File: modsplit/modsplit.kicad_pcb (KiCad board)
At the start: 2 copper layers, 19 x 19 mm, 8 parts, among them J1 Conn_01x04, J2 Conn_01x04, J3 Conn_01x04, J4 Conn_01x04, U1 TRRS, U2 TRRS, U3 TRRS, U4 TRRS

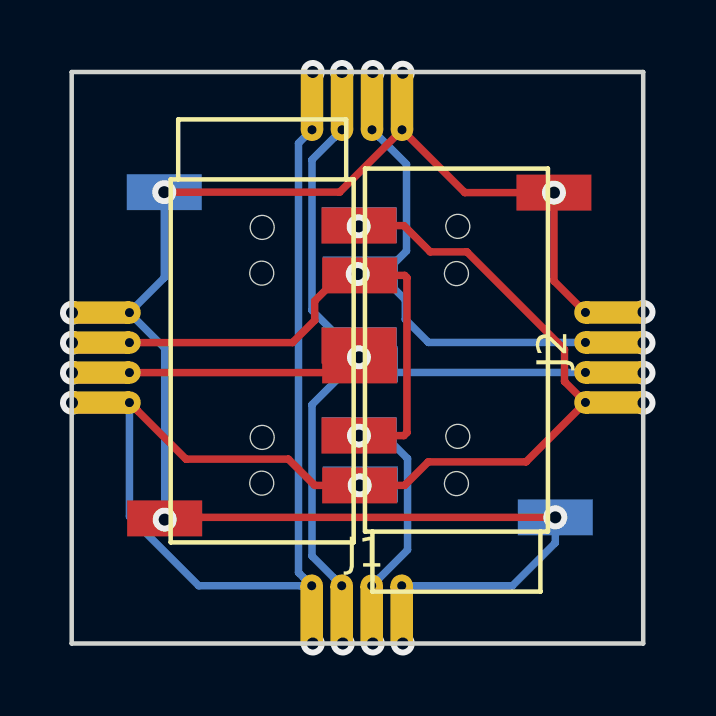
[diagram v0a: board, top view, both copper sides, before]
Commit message: pull up with less than the force of a thousand suns
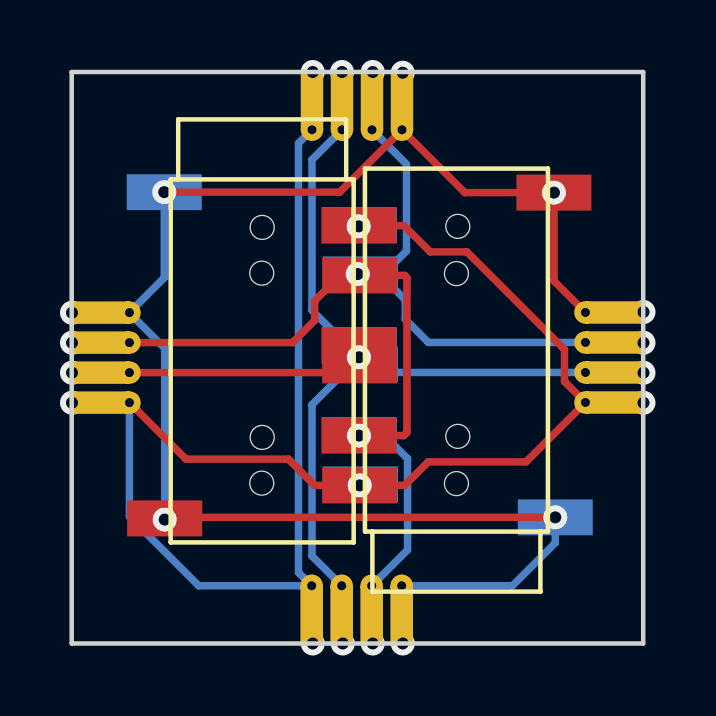
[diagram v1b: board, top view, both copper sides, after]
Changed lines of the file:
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@@
   (module Keebio-Parts:TRRS-PJ-320D (layer B.Cu)
     (at 133.585 89.765 180)
-    (fp_text reference U4 (at 0 -14.2) (layer Dwgs.User)
+    (fp_text reference U4 (at 0 -14.2) (layer Dwgs.User) hide
       (effects (font (size 1 1) (thickness 0.15)))
     )
@@
   (module Keebio-Parts:TRRS-PJ-320D (layer F.Cu)
     (at 133.54 101.54 180)
-    (fp_text reference U3 (at 0 14.2) (layer Dwgs.User)
+    (fp_text reference U3 (at 0 14.2) (layer Dwgs.User) hide
       (effects (font (size 1 1) (thickness 0.15)))
     )
@@
   (module Keebio-Parts:TRRS-PJ-320D (layer F.Cu)
     (at 127.065 89.8)
-    (fp_text reference U2 (at 0 14.2) (layer Dwgs.User)
+    (fp_text reference U2 (at 0 14.2) (layer Dwgs.User) hide
       (effects (font (size 1 1) (thickness 0.15)))
     )
@@
   (module Keebio-Parts:TRRS-PJ-320D (layer B.Cu)
     (at 127.05 101.525)
-    (fp_text reference U1 (at 0 -14.2) (layer Dwgs.User)
+    (fp_text reference U1 (at 0 -14.2) (layer Dwgs.User) hide
       (effects (font (size 1 1) (thickness 0.15)))
     )
@@
   (module modkeeb:edgeconnector (layer B.Cu)
     (at 130.225 86.145)
-    (fp_text reference J4 (at 0.275 3.1 180) (layer B.SilkS)
+    (fp_text reference J4 (at 0.275 3.1 180) (layer B.SilkS) hide
       (effects (font (size 1 1) (thickness 0.15)) (justify mirror))
     )
@@
   (module modkeeb:edgeconnector (layer B.Cu)
     (at 120.64 95.74 90)
-    (fp_text reference J3 (at 0.275 3.1 90) (layer B.SilkS)
+    (fp_text reference J3 (at 0.275 3.1 90) (layer B.SilkS) hide
       (effects (font (size 1 1) (thickness 0.15)) (justify mirror))
     )
@@
   (module modkeeb:edgeconnector (layer F.Cu)
     (at 139.84 95.735 90)
-    (fp_text reference J2 (at 0.275 -3.1 270) (layer F.SilkS)
+    (fp_text reference J2 (at 0.275 -3.1 270) (layer F.SilkS) hide
       (effects (font (size 1 1) (thickness 0.15)))
     )
@@
   (module modkeeb:edgeconnector (layer F.Cu)
     (at 130.215 105.345)
-    (fp_text reference J1 (at 0.275 -3.1 180) (layer F.SilkS)
+    (fp_text reference J1 (at 0.275 -3.1 180) (layer F.SilkS) hide
       (effects (font (size 1 1) (thickness 0.15)))
     )
@@
   (gr_line (start 120.715 105.27) (end 120.715 86.22) (layer Edge.Cuts) (width 0.15))
   (gr_line (start 120.715 86.22) (end 139.765 86.22) (layer Edge.Cuts) (width 0.15))
-  (via (at 130.25 92.955) (size 0.8) (drill 0.4) (layers F.Cu B.Cu) (net 2))
-  (via (at 128.75 86.22) (size 0.8) (drill 0.4) (layers F.Cu B.Cu) (net 4))
-  (via (at 120.725 97.245) (size 0.8) (drill 0.4) (layers F.Cu B.Cu) (net 4))
   (via (at 139.775 94.22) (size 0.8) (drill 0.4) (layers F.Cu B.Cu) (net 1))
   (via (at 131.75 105.27) (size 0.8) (drill 0.4) (layers F.Cu B.Cu) (net 1))
-  (via (at 139.775 95.245) (size 0.8) (drill 0.4) (layers F.Cu B.Cu) (net 2))
-  (via (at 130.75 105.27) (size 0.8) (drill 0.4) (layers F.Cu B.Cu) (net 2))
-  (via (at 120.725 96.245) (size 0.8) (drill 0.4) (layers F.Cu B.Cu) (net 3))
-  (via (at 129.725 86.22) (size 0.8) (drill 0.4) (layers F.Cu B.Cu) (net 3))
-  (via (at 130.75 86.22) (size 0.8) (drill 0.4) (layers F.Cu B.Cu) (net 2))
-  (via (at 120.725 95.245) (size 0.8) (drill 0.4) (layers F.Cu B.Cu) (net 2))
-  (via (at 139.775 96.245) (size 0.8) (drill 0.4) (layers F.Cu B.Cu) (net 3))
-  (via (at 129.75 105.27) (size 0.8) (drill 0.4) (layers F.Cu B.Cu) (net 3))
-  (via (at 128.75 105.27) (size 0.8) (drill 0.4) (layers F.Cu B.Cu) (net 4))
-  (via (at 139.775 97.245) (size 0.8) (drill 0.4) (layers F.Cu B.Cu) (net 4))
   (via (at 120.725 94.245) (size 0.8) (drill 0.4) (layers F.Cu B.Cu) (net 1))
   (via (at 131.75 86.245) (size 0.8) (drill 0.4) (layers F.Cu B.Cu) (net 1))
@@
   (segment (start 123.89 101.065) (end 123.815 101.14) (width 0.25) (layer F.Cu) (net 1))
   (segment (start 136.835 101.065) (end 123.89 101.065) (width 0.25) (layer F.Cu) (net 1))
+  (via (at 130.25 92.955) (size 0.8) (drill 0.4) (layers F.Cu B.Cu) (net 2))
+  (via (at 139.775 95.245) (size 0.8) (drill 0.4) (layers F.Cu B.Cu) (net 2))
+  (via (at 130.75 105.27) (size 0.8) (drill 0.4) (layers F.Cu B.Cu) (net 2))
+  (via (at 130.75 86.22) (size 0.8) (drill 0.4) (layers F.Cu B.Cu) (net 2))
+  (via (at 120.725 95.245) (size 0.8) (drill 0.4) (layers F.Cu B.Cu) (net 2))
   (segment (start 131.875001 89.295001) (end 130.988888 88.408888) (width 0.25) (layer B.Cu) (net 2))
   (segment (start 130.988888 88.408888) (end 130.725 88.145) (width 0.25) (layer B.Cu) (net 2))
@@
   (segment (start 131.130002 98.325) (end 131.910001 99.104999) (width 0.25) (layer B.Cu) (net 2))
   (segment (start 130.3 98.325) (end 131.130002 98.325) (width 0.25) (layer B.Cu) (net 2))
+  (via (at 120.725 96.245) (size 0.8) (drill 0.4) (layers F.Cu B.Cu) (net 3))
+  (via (at 129.725 86.22) (size 0.8) (drill 0.4) (layers F.Cu B.Cu) (net 3))
+  (via (at 139.775 96.245) (size 0.8) (drill 0.4) (layers F.Cu B.Cu) (net 3))
+  (via (at 129.75 105.27) (size 0.8) (drill 0.4) (layers F.Cu B.Cu) (net 3))
   (segment (start 130.36 96.235) (end 130.29 96.165) (width 0.25) (layer B.Cu) (net 3))
   (segment (start 137.84 96.235) (end 130.36 96.235) (width 0.25) (layer B.Cu) (net 3))
@@
   (segment (start 128.724999 94.164999) (end 128.724999 89.145001) (width 0.25) (layer B.Cu) (net 3))
   (segment (start 130.29 95.73) (end 128.724999 94.164999) (width 0.25) (layer B.Cu) (net 3))
+  (via (at 128.75 86.22) (size 0.8) (drill 0.4) (layers F.Cu B.Cu) (net 4))
+  (via (at 120.725 97.245) (size 0.8) (drill 0.4) (layers F.Cu B.Cu) (net 4))
+  (via (at 128.75 105.27) (size 0.8) (drill 0.4) (layers F.Cu B.Cu) (net 4))
+  (via (at 139.775 97.245) (size 0.8) (drill 0.4) (layers F.Cu B.Cu) (net 4))
   (via (at 130.28 91.365) (size 0.8) (drill 0.4) (layers F.Cu B.Cu) (net 4))
   (segment (start 137.141796 96.536796) (end 137.84 97.235) (width 0.25) (layer F.Cu) (net 4))
